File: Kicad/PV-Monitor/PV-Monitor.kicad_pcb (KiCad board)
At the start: 2 copper layers, 30 parts, among them J1 Charge Controller, J2 Devices, U1 LM7805_TO220, U2 ACS758LCB-050B, U3 ACS758LCB-050B, U4 ACS758LCB-050B

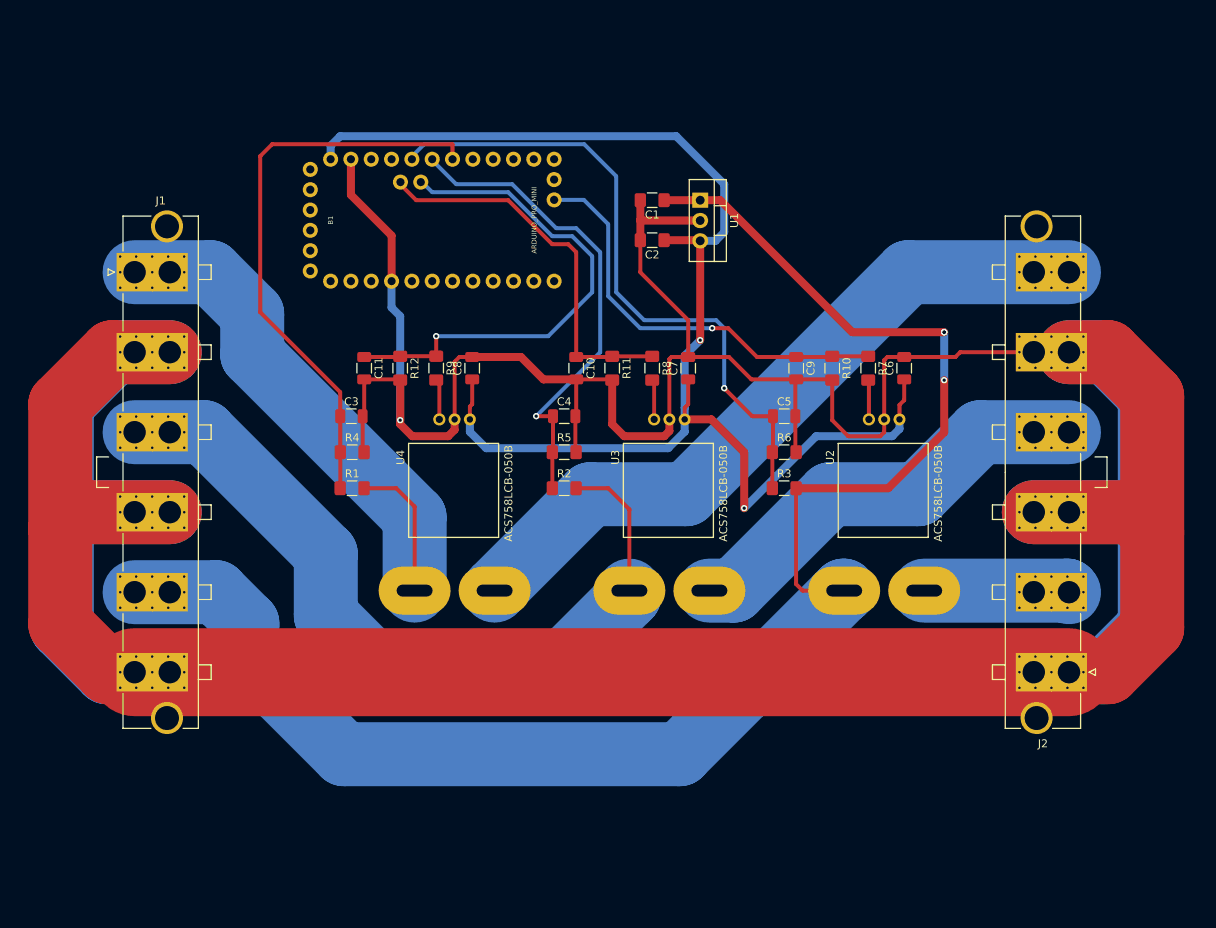
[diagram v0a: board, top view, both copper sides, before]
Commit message: Updates
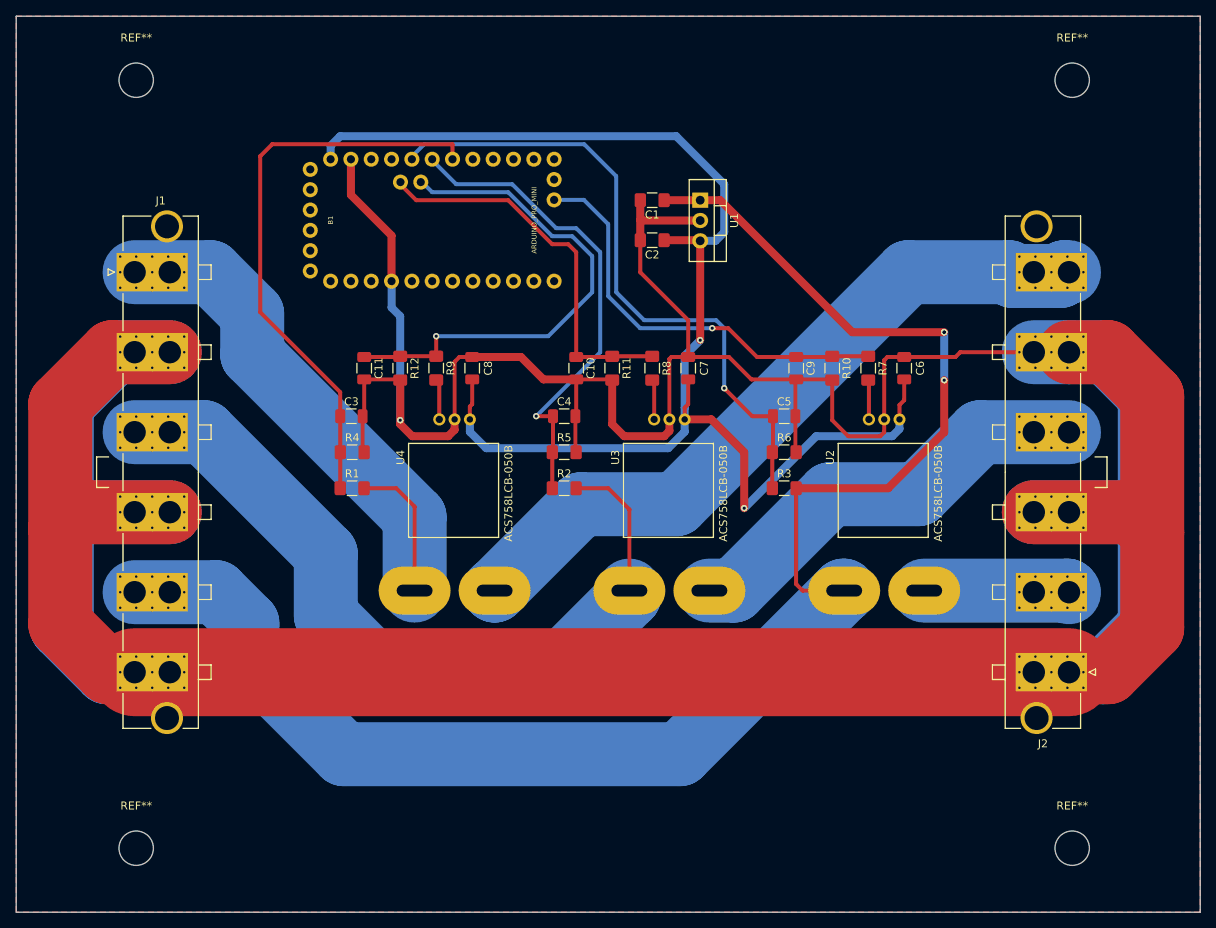
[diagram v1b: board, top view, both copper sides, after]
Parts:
- added REF**: MountingHole_4.3mm_M4, MountingHole:MountingHole_4.3mm_M4, F.Cu at (201.0, 50.0)
- added REF**: MountingHole_4.3mm_M4, MountingHole:MountingHole_4.3mm_M4, F.Cu at (84.0, 50.0)
- added REF**: MountingHole_4.3mm_M4, MountingHole:MountingHole_4.3mm_M4, F.Cu at (84.0, 146.0)
- added REF**: MountingHole_4.3mm_M4, MountingHole:MountingHole_4.3mm_M4, F.Cu at (201.0, 146.0)
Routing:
- net GND: track 624.6 -> 633.6 mm
- added copper zone on F.Cu, net GND
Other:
- board outline added: 148 x 112 mm
